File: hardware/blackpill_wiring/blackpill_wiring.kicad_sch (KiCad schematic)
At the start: 7 parts, among them J1 ST7789_DISPLAY, J2 HOBBY_SERVO, J3 CRSF_RECEIVER, J4 BRUSHLESS_ESC, J5 ESP01_WIFI, J6 USB_HOST, U1 BLACKPILL_F411CE

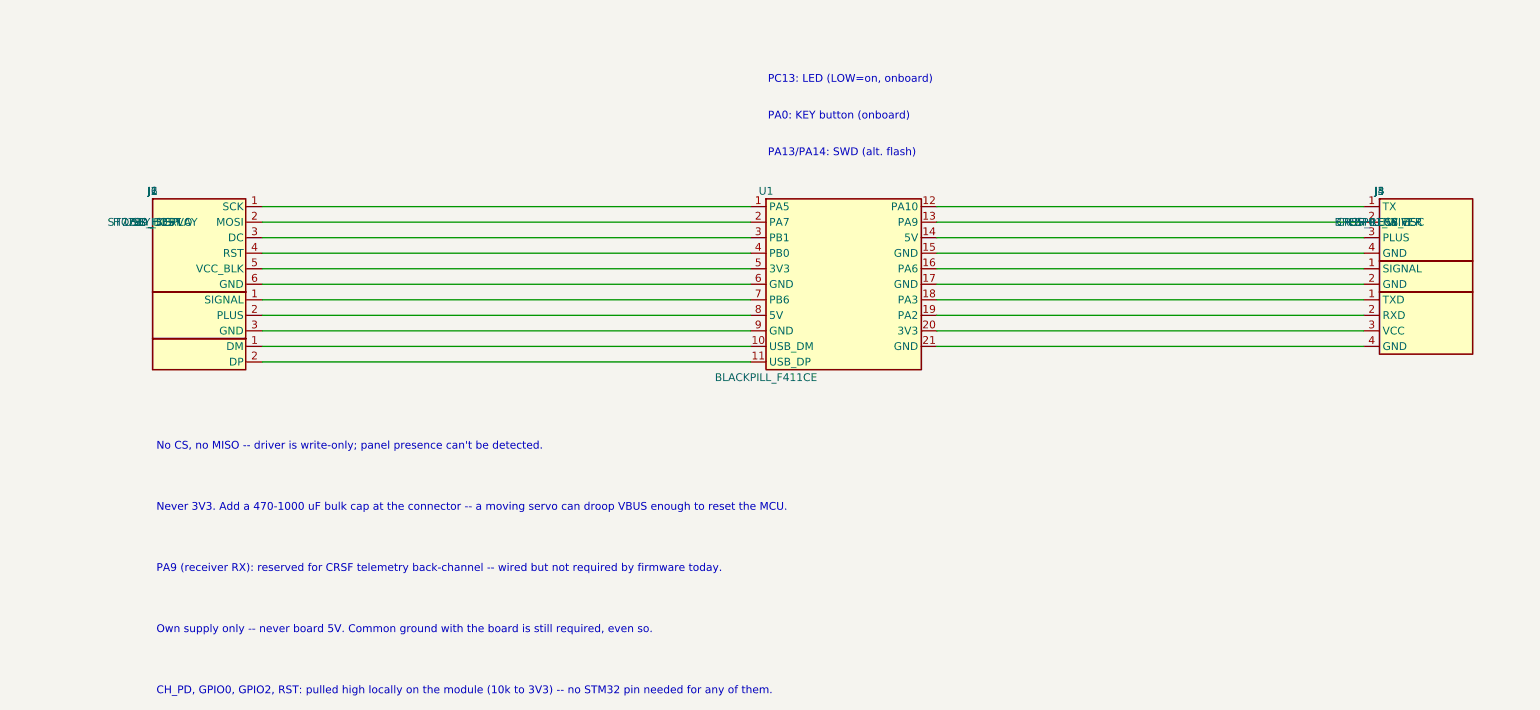
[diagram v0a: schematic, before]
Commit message: modified wiring diags
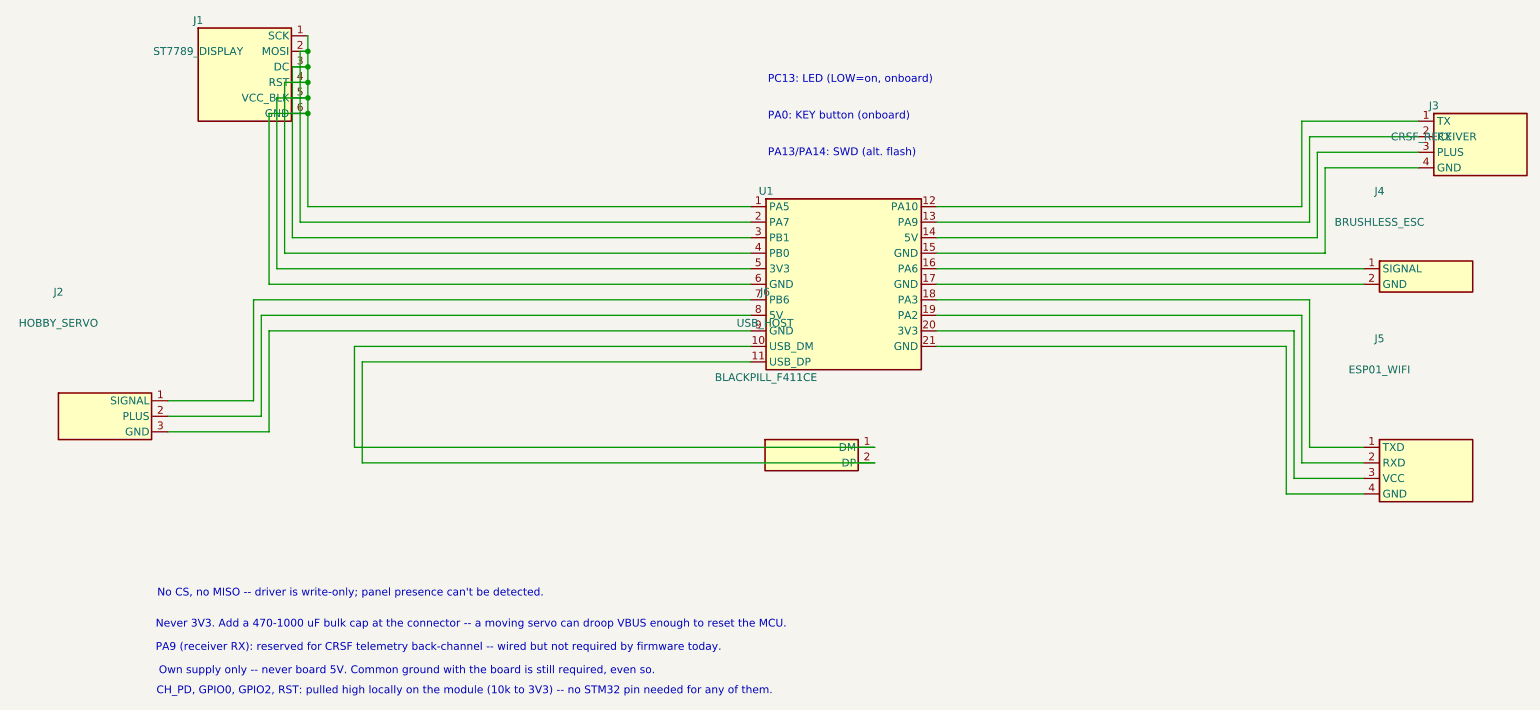
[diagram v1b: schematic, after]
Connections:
- net at J1.1 (SCK), U1.1 (PA5): now also J1.2 (MOSI), J1.3 (DC), J1.4 (RST), J1.5 (VCC_BLK), J1.6 (GND), U1.2 (PA7), U1.3 (PB1), U1.4 (PB0), U1.5 (3V3), U1.6 (GND)
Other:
- moved on the sheet: J1, J2, J3, J5, J6
